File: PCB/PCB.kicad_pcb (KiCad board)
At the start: 2 copper layers, 68 x 17 mm, 52 parts, among them J1 GPIO/Control, J10 OUTPUT1, J2 POWER, J3 OUTPUT2, J4 OUTPUT1, J5 OUTPUT2, J6 OUTPUT1, J7 OUTPUT2, J8 OUTPUT1, J9 OUTPUT2

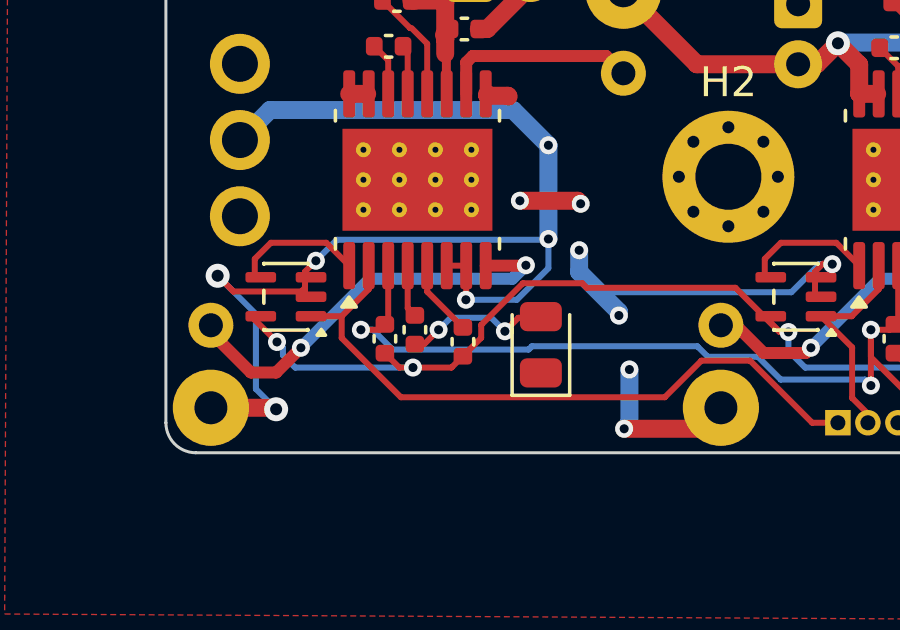
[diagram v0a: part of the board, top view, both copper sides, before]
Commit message: commit
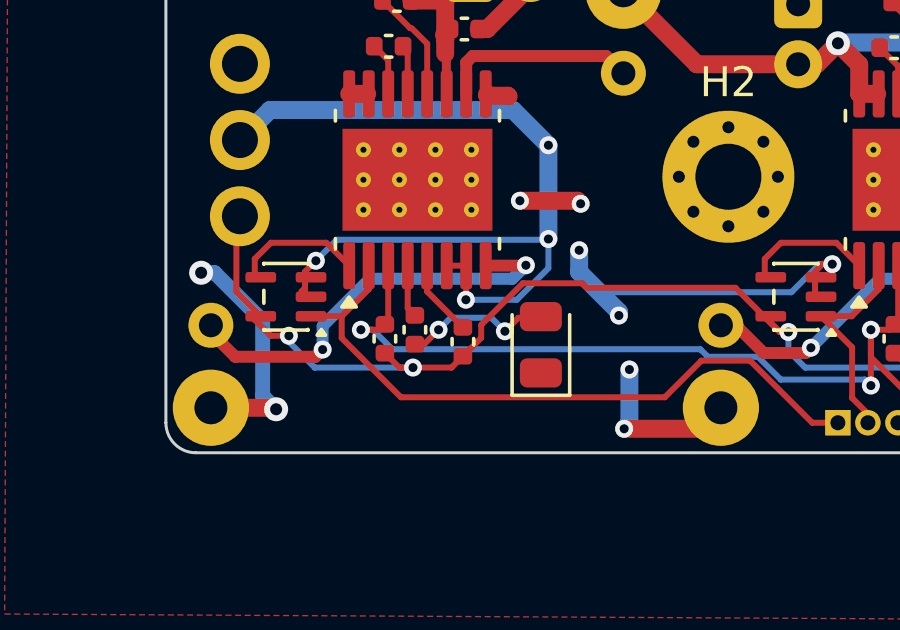
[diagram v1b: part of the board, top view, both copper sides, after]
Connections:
- C2 pad 1: +24V -> +12V
- C3 pad 2: +24V -> +12V
- C4 pad 2: +24V -> +12V
- J2 pad 3: +24V -> +12V
- U1 pad 11: +24V -> +12V
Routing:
- net +12V: track 0.00 -> 11.3 mm, vias 0 -> 2
- net +24V: track 41.6 -> 30.3 mm, vias 2 -> 0
- net +3V3: track 88.3 -> 91.8 mm
- net GND: track 163.7 -> 161.2 mm
- added copper zone on B.Cu, net +12V
- removed copper zone on B.Cu, net +24V
